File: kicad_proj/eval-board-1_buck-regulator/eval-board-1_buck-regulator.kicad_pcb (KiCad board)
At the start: 4 copper layers, 107 x 43 mm, 45 parts, among them J1 Conn_01x02, J2 Conn_01x06, J3 Conn_01x02, U1 SIC453ED-T1-GE3

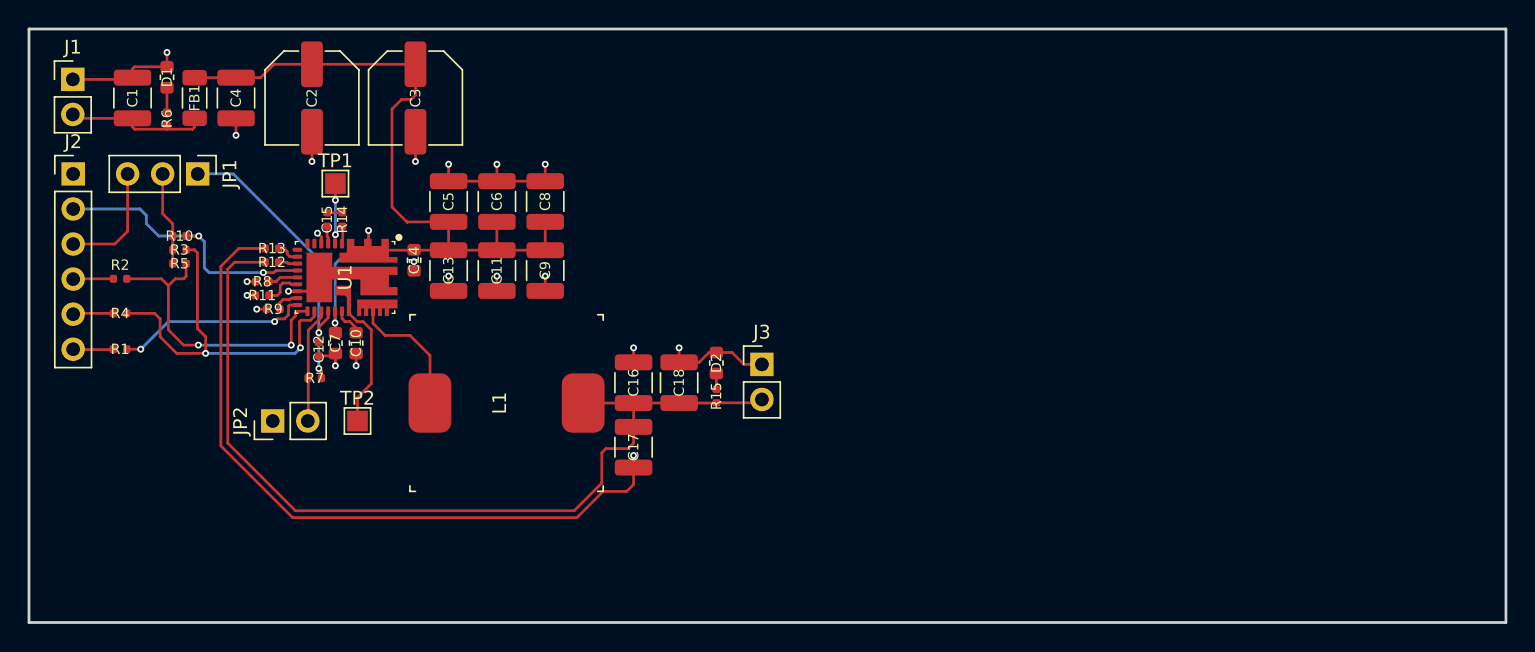
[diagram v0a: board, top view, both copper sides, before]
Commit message: Livestream updates
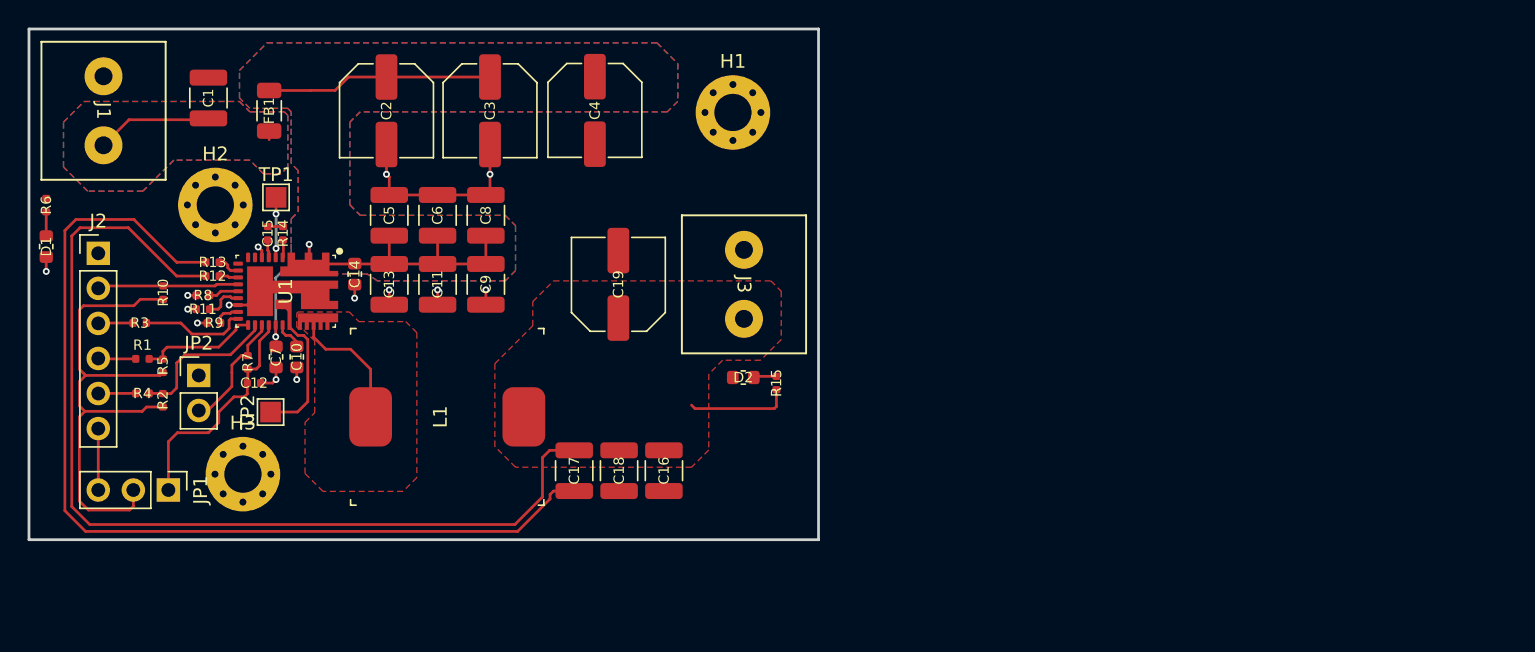
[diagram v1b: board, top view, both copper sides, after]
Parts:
- added C19: UCH1V470MCS1GS, eval-board-1_buck-regulator:CAPAE660X580L260X65N, F.Cu at (42.7, 18.5)
- added H1: MountingHole_Pad, MountingHole:MountingHole_2.7mm_M2.5_Pad_Via, F.Cu at (51.0, 6.05)
- added H2: MountingHole_Pad, MountingHole:MountingHole_2.7mm_M2.5_Pad_Via, F.Cu at (13.5, 12.8)
- added H3: MountingHole_Pad, MountingHole:MountingHole_2.7mm_M2.5_Pad_Via, F.Cu at (15.5, 32.2)
- C4: value GRM32ER71C226KEA8 -> UCH1V470MCS1GS; footprint eval-board-1_buck-regulator:CAPACITOR_1210N -> eval-board-1_buck-regulator:CAPAE660X580L260X65N
- J1, J3: footprint Connector_PinHeader_2.54mm:PinHeader_1x02_P2.54mm_Vertical -> eval-board-1_buck-regulator:1935776
- moved C4 26.0 mm to (41.0, 5.90)
- moved JP1 23.0 mm to (10.1, 33.4)
- moved D1 15.1 mm to (1.25, 15.8), turned to 90 degrees
- moved R2 11.0 mm to (9.70, 26.9), turned to 90 degrees
- moved R6 10.8 mm to (1.25, 12.8), turned to -90 degrees
- moved C18 7.72 mm to (42.8, 32.0), turned to -90 degrees
- moved R5 7.50 mm to (9.70, 24.4), turned to 90 degrees
- moved C16 6.74 mm to (46.0, 32.0), turned to -90 degrees
- moved TP2 6.33 mm to (17.5, 27.8), turned to 90 degrees
- moved JP2 6.29 mm to (12.3, 25.1), turned to 0 degrees
- moved J2 6.03 mm to (5.02, 16.2)
- moved R1 6.02 mm to (8.22, 23.9)
- moved R4 6.02 mm to (8.22, 26.4)
- moved J3 5.94 mm to (51.8, 18.5), turned to -90 degrees
- moved C1 5.50 mm to (13.0, 5.00)
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- renumbered R2 to R1, R3 to R2, R1 to R3
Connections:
- J2 pad 3: /EXTERN_VTG -> Net-(J2-Pad3)
- J2 pad 6: Net-(J2-Pad6) -> /EXTERN_VTG
- R3 pad 1: Net-(J2-Pad6) -> Net-(J2-Pad3)
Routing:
- net /PULLUP_VTG: track 6.80 -> 37.9 mm
- net Net-(C11-Pad1): track 63.6 -> 47.5 mm
- net /SCL: track 26.7 -> 11.0 mm, vias 2 -> 0
- net +5V: track 66.2 -> 79.4 mm
- net /SDA: track 21.6 -> 8.67 mm, vias 2 -> 0
- net /PGOOD: track 20.6 -> 10.7 mm, vias 2 -> 0
- net /SALERT: track 14.0 -> 7.78 mm, vias 2 -> 0
- net /VDD: track 22.6 -> 17.1 mm, vias 2 -> 0
- net /EXTERN_VTG: track 8.48 -> 4.52 mm
- net Net-(J2-Pad6): track 2.90 -> 0.00 mm
- net Net-(J2-Pad3): track 0.00 -> 2.53 mm
- net GND: track 101.5 -> 103.2 mm, vias 21 -> 14
- net +12V: track 10.3 -> 8.90 mm
- net Net-(D2-Pad2): track 1.15 -> 1.68 mm
- added copper zone on B.Cu, net +12V
- added copper zone on F.Cu, net +12V
- added copper zone on F.Cu, net +5V
- added copper zone on B.Cu, net Net-(C11-Pad1)
- added copper zone on F.Cu, net Net-(C11-Pad1)
- added copper zone on F.Cu, net Net-(L1-Pad1)
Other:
- board size 107 x 43 mm -> 57.2 x 37 mm
